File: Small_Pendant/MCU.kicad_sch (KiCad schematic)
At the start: 33 parts, among them J1 USB_C_Receptacle_USB2.0_16P, U1 FT234XD-R, U2 SN74LVC1T45DCK, U3 ESP32-C3-MINI-1

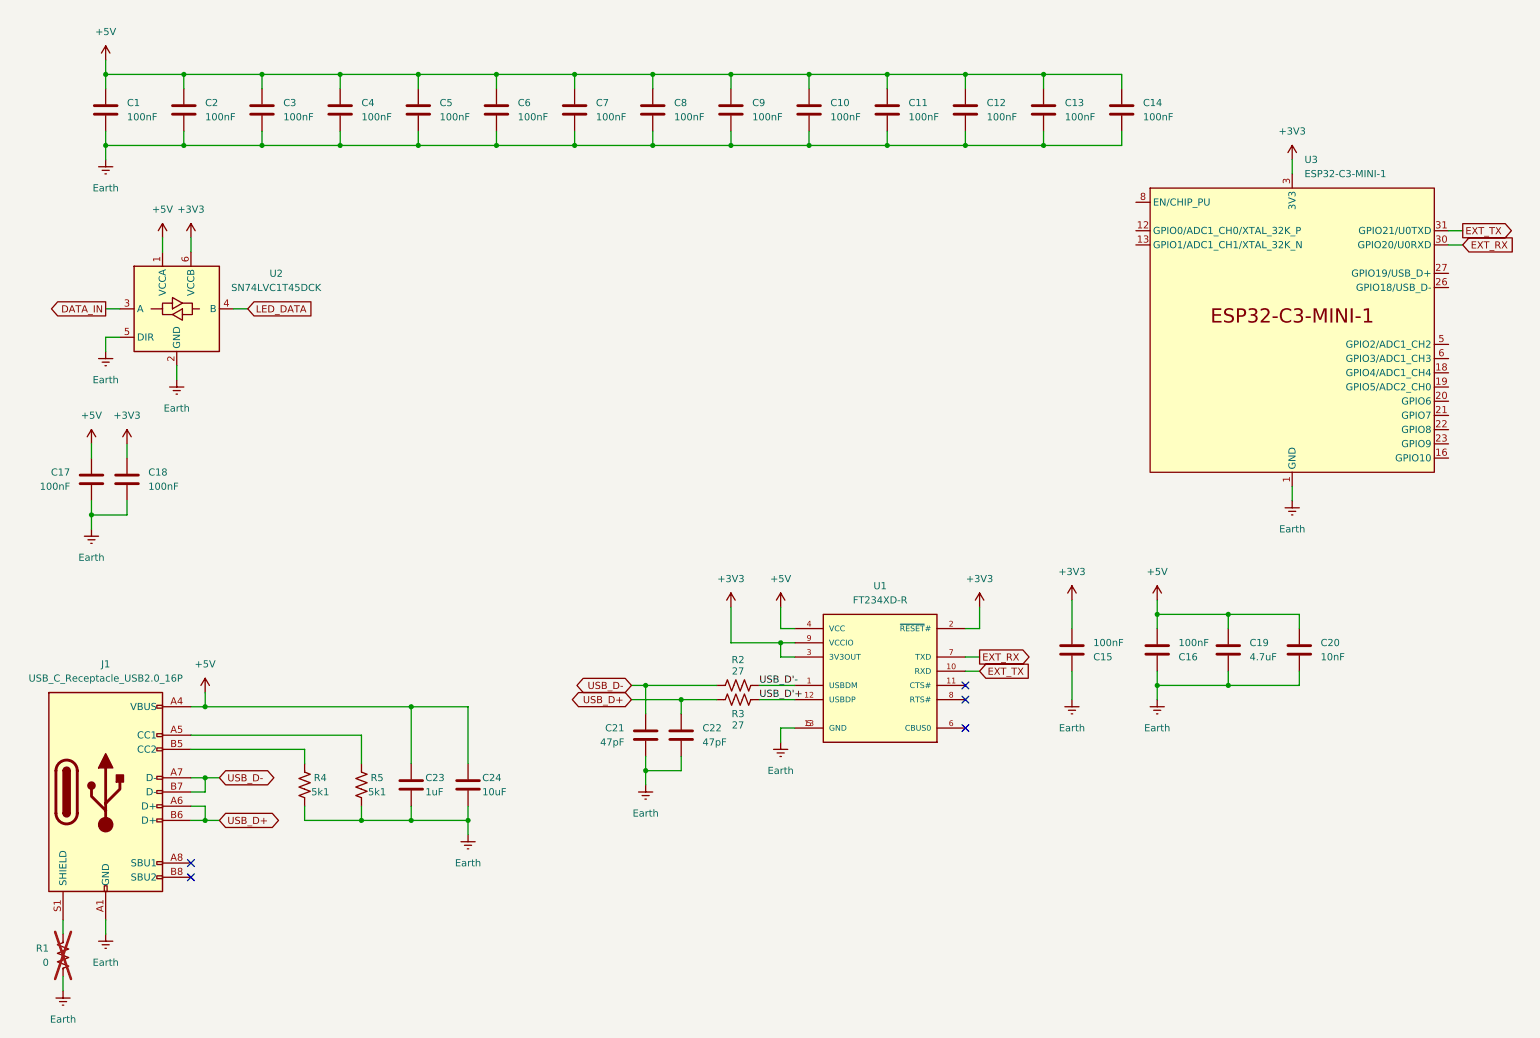
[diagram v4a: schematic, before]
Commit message: [HW] Added IMU and corrected UART Bridge, all chip support components added, still need reset and boot connections though
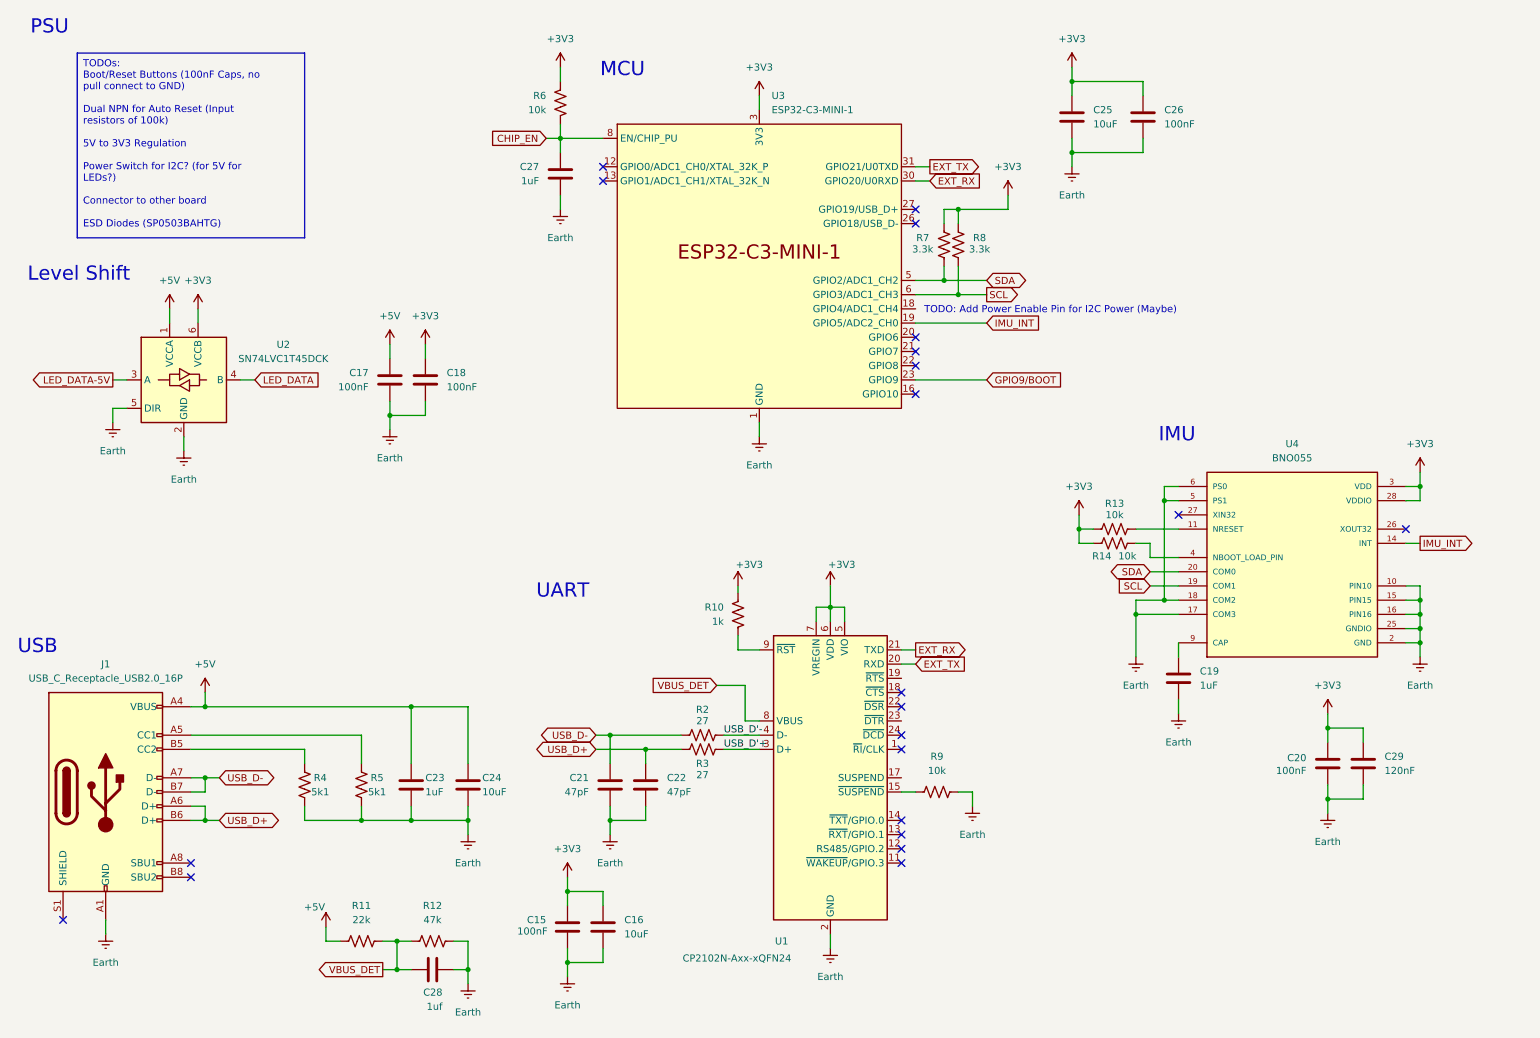
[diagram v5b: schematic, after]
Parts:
- removed C1, C10, C11, C12, C13, C14, C2, C3, C4, C5, C6, C7, C8, C9: 100nF, Capacitor_SMD:C_0402_1005Metric, symbol Device:C
- removed R1: 0, Resistor_SMD:R_0402_1005Metric, symbol Device:R_US
- removed U1: FT234XD-R, Package_DFN_QFN:DFN-12-1EP_3x3mm_P0.45mm_EP1.65x2.38mm, symbol Interface_USB:FT234XD-R
- added C25: 10uF, Capacitor_SMD:C_0402_1005Metric, symbol Device:C
- added C26: 100nF, Capacitor_SMD:C_0402_1005Metric, symbol Device:C
- added C27: 1uF, Capacitor_SMD:C_0402_1005Metric, symbol Device:C
- added C28: 1uf, Capacitor_SMD:C_0402_1005Metric, symbol Device:C
- added C29: 120nF, Capacitor_SMD:C_0402_1005Metric, symbol Device:C
- added R10: 1k, Resistor_SMD:R_0402_1005Metric, symbol Device:R_US
- added R11: 22k, Resistor_SMD:R_0402_1005Metric, symbol Device:R_US
- added R12: 47k, Resistor_SMD:R_0402_1005Metric, symbol Device:R_US
- added R13, R14, R6, R9: 10k, Resistor_SMD:R_0402_1005Metric, symbol Device:R_US
- added R7, R8: 3.3k, Resistor_SMD:R_0402_1005Metric, symbol Device:R_US
- added U1: CP2102N-Axx-xQFN24, Package_DFN_QFN:QFN-24-1EP_4x4mm_P0.5mm_EP2.6x2.6mm, symbol Interface_USB:CP2102N-Axx-xQFN24
- added U4: BNO055, BNO055:LGA28R50P4X10_380X520X100, symbol BNO055:BNO055
- C16: value 100nF -> 10uF
- C19: value 4.7uF -> 1uF
- C20: value 10nF -> 100nF
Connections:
- net +3V3: now also C16.1, C20.2, C25.1, C26.1, C29.1, R10.1, R13.1, R14.1, R6.1, R7.2, R8.2, U1.5 (VIO), U1.6 (VDD), U1.7 (VREGIN), U4.28 (VDDIO), U4.3 (VDD)
- net +5V: now also R11.2; no longer C16.2, C19.1, C20.1
- net EXT_RX: now also U1.21 (TXD)
- net EXT_TX: now also U1.20 (RXD)
- net Earth: now also C16.2, C20.1, C25.2, C26.2, C27.2, C28.2, C29.2, R12.2, R9.2, U1.2 (GND), U1.25 (GND), U4.10 (PIN10), U4.15 (PIN15), U4.16 (PIN16), U4.17 (COM3), U4.18 (COM2), U4.2 (GND), U4.25 (GNDIO), U4.5 (PS1), U4.6 (PS0); no longer C16.1, C20.2
- net USB_D'+: now also U1.3 (D+)
- net USB_D'-: now also U1.4 (D-)
- net IMU_INT: now reaches U3.19 (GPIO5/ADC2_CH0)
- net IMU_INT: now also U4.14 (INT)
- net GPIO9/BOOT: now reaches U3.23 (GPIO9)
- net SDA: now reaches U3.5 (GPIO2/ADC1_CH2)
- net SDA: now also R7.1, U4.20 (COM0)
- net SCL: now reaches U3.6 (GPIO3/ADC1_CH3)
- net SCL: now also R8.1, U4.19 (COM1)
- net CHIP_EN: now reaches U3.8 (EN/CHIP_PU)
- net CHIP_EN: now also C27.1, R6.2
- net DATA_IN renamed LED_DATA-5V
- new net: R10.2, U1.9 (~{RST})
- new net: R13.2, U4.11 (NRESET)
- new net: R9.1, U1.15 (~{SUSPEND})
- new net: C19.1, U4.9 (CAP)
- new net: R14.2, U4.4 (NBOOT_LOAD_PIN)
- new net: U4.1 (PIN1), U4.12 (PIN12), U4.13 (PIN13), U4.21 (PIN21), U4.22 (PIN22), U4.23 (PIN23), U4.24 (PIN24)
- new net VBUS_DET: C28.1, R11.1, R12.1, U1.8 (VBUS)
- no-connect marks 5 -> 21
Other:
- note added: "IMU"
- note added: "Level Shift"
- note added: "MCU"
- note added: "PSU"
- note added: "TODO: Add Power Enable Pin for I2C Power (Maybe)"
- note added: "UART"
- note added: "USB"
- moved on the sheet: C15, C17, C18, C21, C22, R2, R3, U2, U3

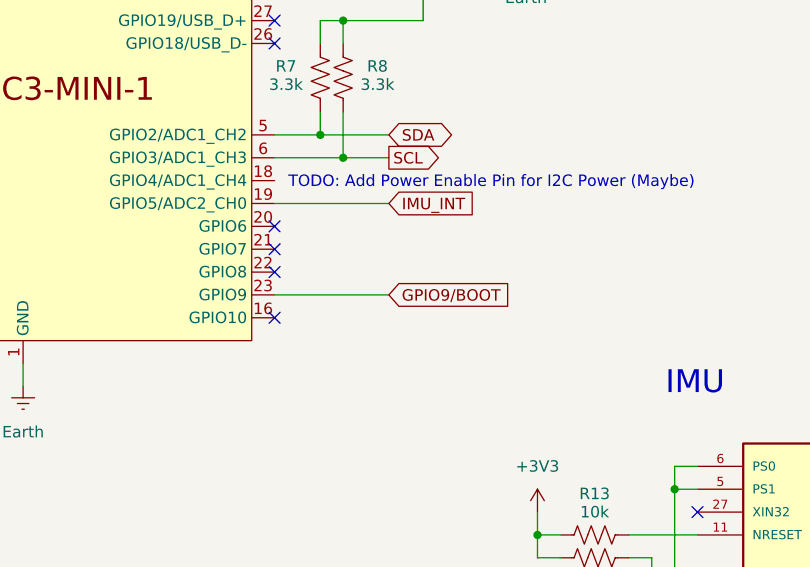
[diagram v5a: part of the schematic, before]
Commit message: [HW] Move Support Components in
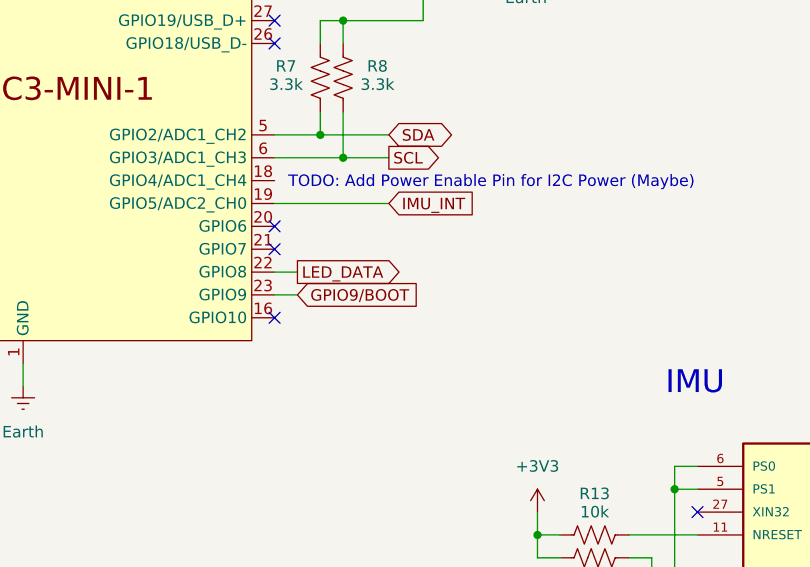
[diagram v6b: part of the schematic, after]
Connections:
- net LED_DATA: now also U3.22 (GPIO8)
- no-connect marks 21 -> 20
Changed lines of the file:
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@@
-	)
-	(no_connect
-		(at 175.26 77.47)
 	)
 	(no_connect
@@
 	(wire
 		(pts
+			(xy 175.26 77.47) (xy 177.8 77.47)
+		)
+		(stroke
+			(width 0)
+			(type default)
+		)
+	)
+	(wire
+		(pts
 			(xy 222.25 139.7) (xy 222.25 137.16)
 		)
@@
 	(wire
 		(pts
-			(xy 175.26 80.01) (xy 187.96 80.01)
+			(xy 175.26 80.01) (xy 177.8 80.01)
 		)
 		(stroke
@@
 	(global_label "GPIO9{slash}BOOT"
 		(shape input)
-		(at 187.96 80.01 0)
+		(at 177.8 80.01 0)
 		(fields_autoplaced yes)
 		(effects
@@
 		)
 		(property "Intersheetrefs" "${INTERSHEET_REFS}"
-			(at 202.8591 80.01 0)
+			(at 192.6991 80.01 0)
 			(effects
 				(font
@@
 				(hide yes)
 			)
+		)
+	)
+	(global_label "LED_DATA"
+		(shape output)
+		(at 177.8 77.47 0)
+		(fields_autoplaced yes)
+		(effects
+			(font
+				(size 1.27 1.27)
+			)
+			(justify left)
+		)
+		(property "Intersheetrefs" "${INTERSHEET_REFS}"
+			(at 189.6147 77.47 0)
+			(effects
+				(font
+					(size 1.27 1.27)
+				)
+				(justify left)
+				(hide yes)
+			)

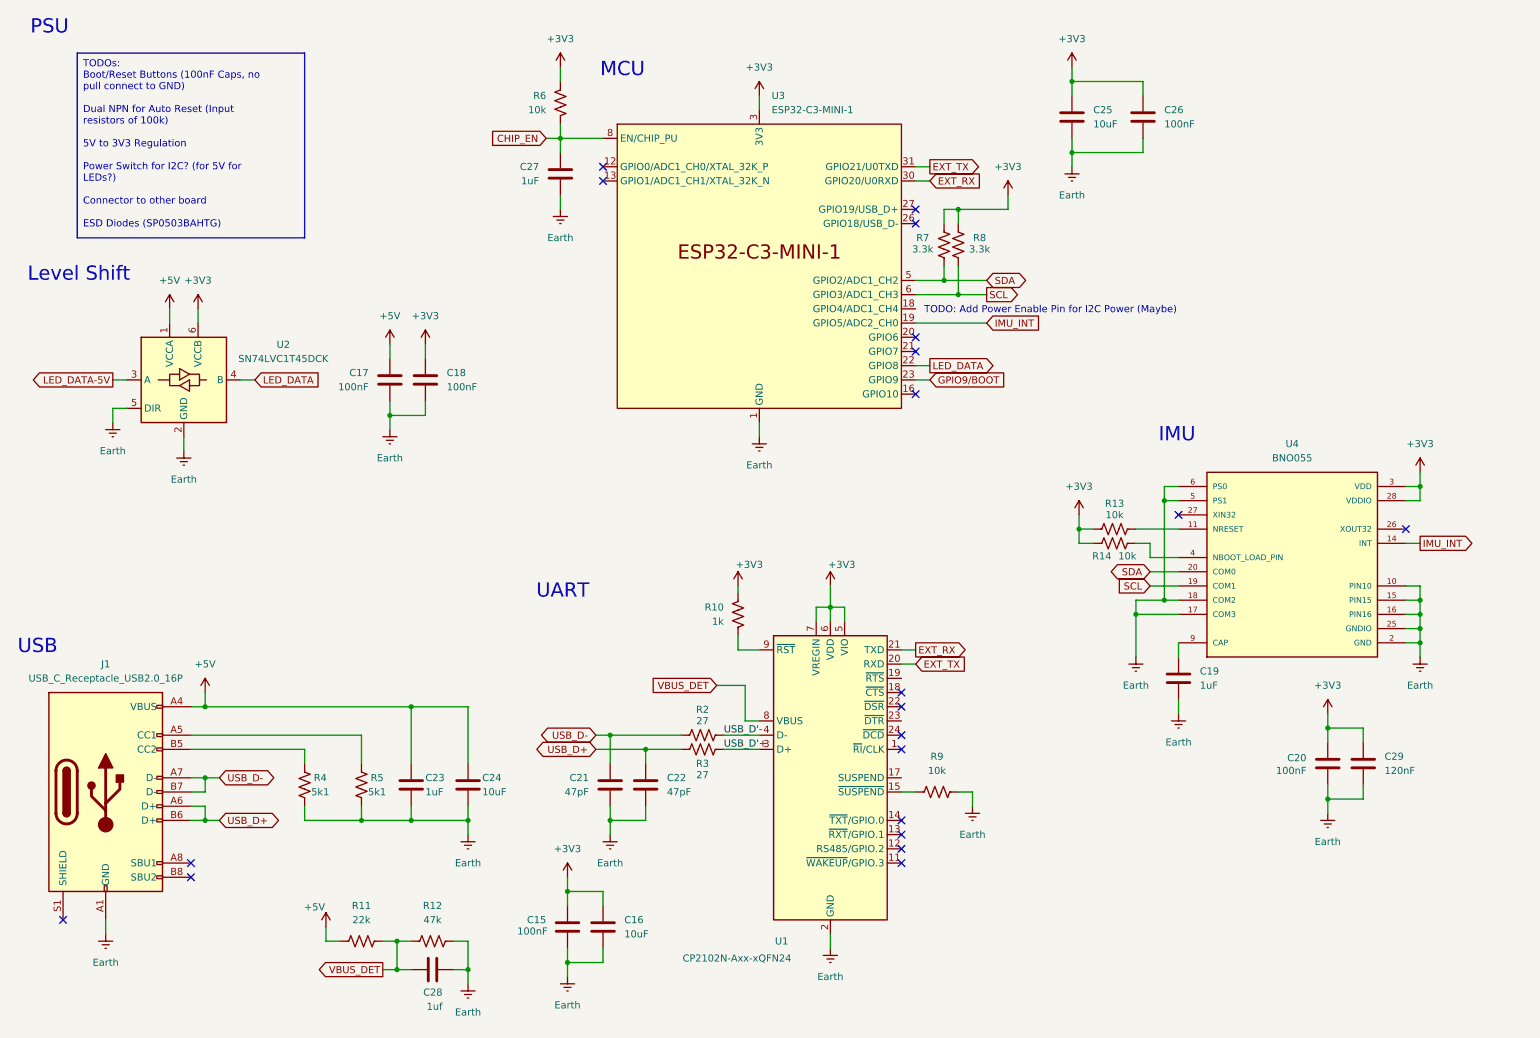
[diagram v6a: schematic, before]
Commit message: [HW] Add Buttons and Replace Transistors Picked a Connector, need to create symbol and footprint Need VREG, then that's all components Still lots of DRC issues
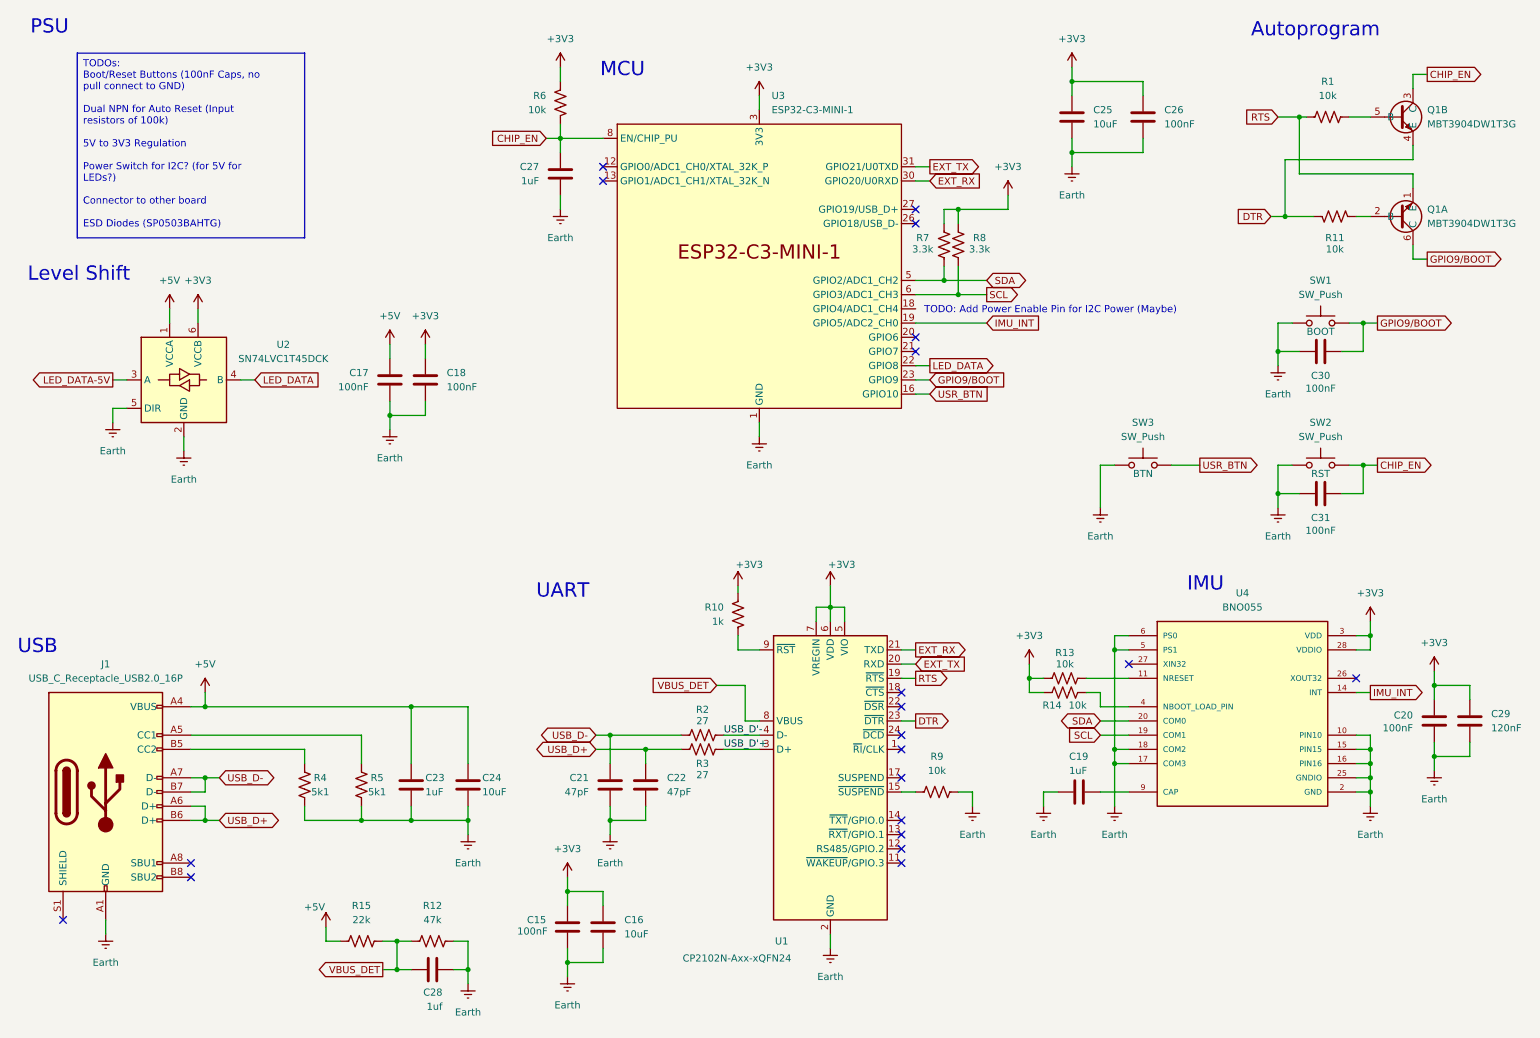
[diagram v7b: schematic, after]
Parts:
- added C30, C31: 100nF, Capacitor_SMD:C_0402_1005Metric, symbol Device:C
- added Q1: MBT3904DW1T3G, EasyEDA2KiCad:SOT-363-6_L2.2-W1.3-P0.65-LS2.1-BL, symbol EasyEDA2KiCad:MBT3904DW1T3G
- added R1, R11: 10k, Resistor_SMD:R_0402_1005Metric, symbol Device:R_US
- added SW1, SW2, SW3: SW_Push, EasyEDA2KiCad:KEY-SMD_L3.9-W3.0-LS5.0-EH, symbol Switch:SW_Push
- J1: Part# (none) -> C3020560
- U1: Part# (none) -> C969151
- U2: Part# (none) -> C9382
- U3: Part# (none) -> C2934569
- U4: Part# (none) -> C93216
- renumbered R11 to R15
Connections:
- net CHIP_EN: now also C31.1, Q1.3 (C), SW2.2
- net Earth: now also C30.2, C31.2, SW1.1, SW2.1, SW3.1
- net GPIO9/BOOT: now also C30.1, Q1.6 (C), SW1.2
- net RTS: now reaches U1.19 (~{RTS})
- net RTS: now also Q1.1 (E), R1.1
- net DTR: now reaches U1.23 (~{DTR})
- net DTR: now also Q1.4 (E), R11.1
- net USR_BTN: now reaches U3.16 (GPIO10)
- net USR_BTN: now also SW3.2
- new net: Q1.5 (B), R1.2
- new net: Q1.2 (B), R11.2
- now unconnected: U4.1 (PIN1), U4.12 (PIN12), U4.13 (PIN13), U4.21 (PIN21), U4.22 (PIN22), U4.23 (PIN23), U4.24 (PIN24)
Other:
- note added: "Autoprogram"
- moved on the sheet: C19, C20, C29, R13, R14, U4
